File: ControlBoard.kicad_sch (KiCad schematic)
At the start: 1 part

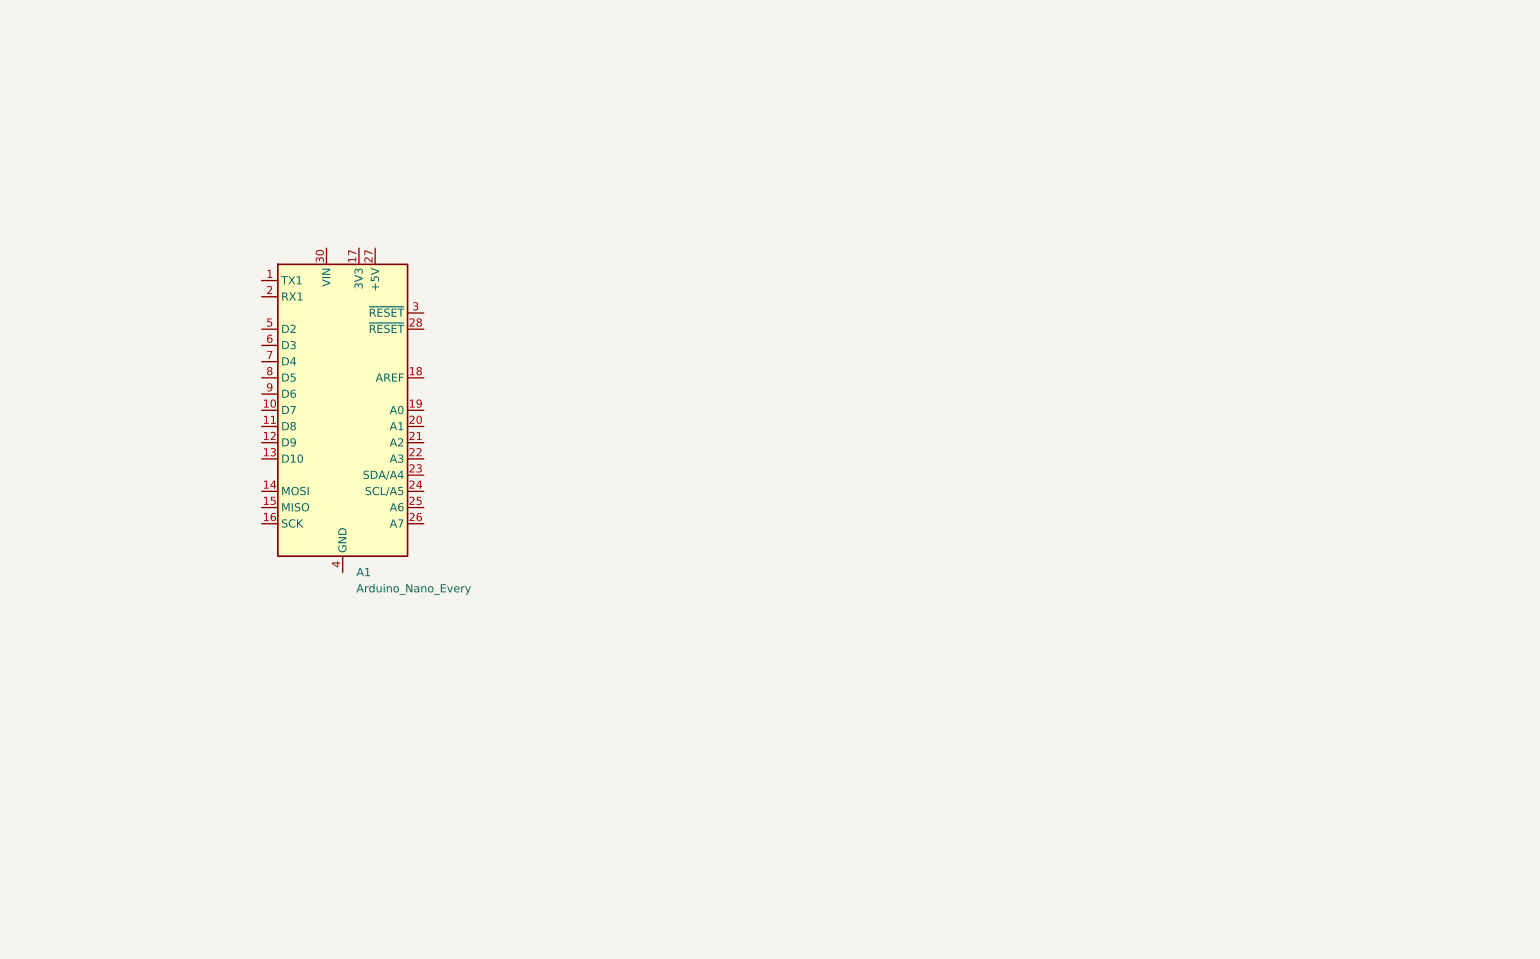
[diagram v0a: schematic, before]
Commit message: sync
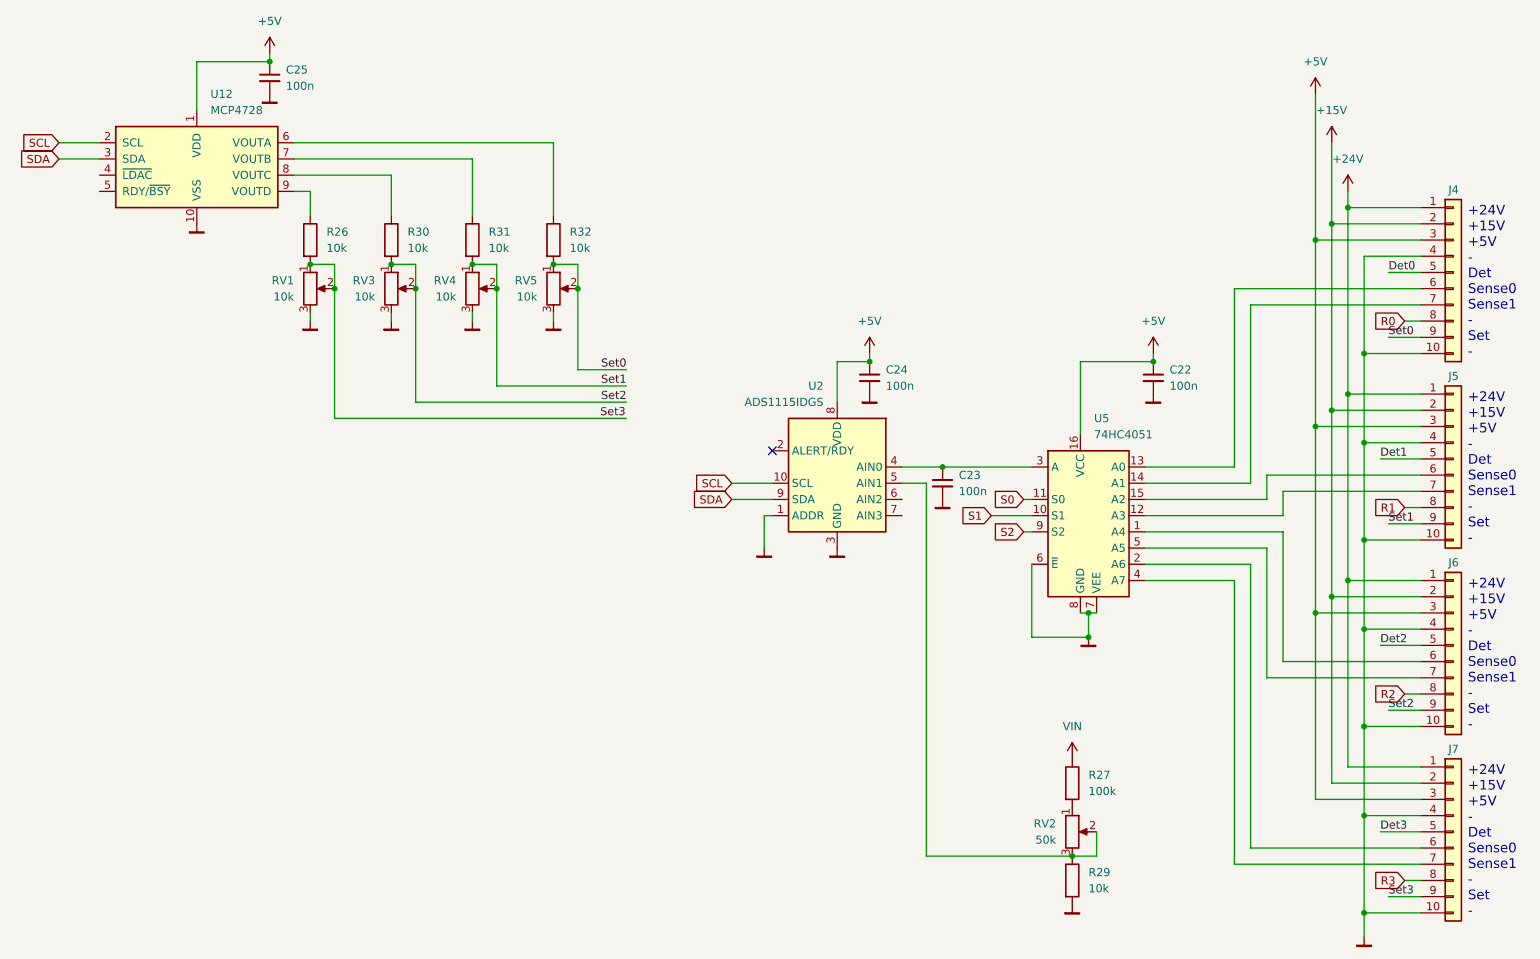
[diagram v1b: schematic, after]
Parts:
- removed A1: Arduino_Nano_Every, Module:Arduino_Nano, symbol MCU_Module:Arduino_Nano_Every
- added C22, C23, C24, C25: 100n, Capacitor_SMD:C_0603_1608Metric, symbol Device:C_Small
- added J4, J5, J6, J7: Conn_01x10, Connector_PinHeader_2.54mm:PinHeader_1x10_P2.54mm_Vertical, symbol Connector_Generic:Conn_01x10
- added R26, R29, R30, R31, R32: 10k, Resistor_SMD:R_0603_1608Metric, symbol Device:R
- added R27: 100k, Resistor_SMD:R_0603_1608Metric, symbol Device:R
- added RV1, RV3, RV4, RV5: 10k, Potentiometer_THT:Potentiometer_ACP_CA14-H5_Horizontal, symbol Device:R_Potentiometer
- added RV2: 50k, Potentiometer_THT:Potentiometer_ACP_CA14-H4_Horizontal, symbol Device:R_Potentiometer
- added U12: MCP4728, Package_SO:MSOP-10_3x3mm_P0.5mm, symbol Analog_DAC:MCP4728
- added U2: ADS1115IDGS, Package_SO:TSSOP-10_3x3mm_P0.5mm, symbol Analog_ADC:ADS1115IDGS
- added U5: 74HC4051, Package_SO:SOIC-16_3.9x9.9mm_P1.27mm, symbol 74xx:74HC4051
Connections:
- new net: J7.6 (Pin_6), U5.2 (A6)
- new net: J7.7 (Pin_7), U5.4 (A7)
- new net: R30.1, U12.8 (VOUTC)
- new net: R31.1, U12.7 (VOUTB)
- new net: R32.1, U12.6 (VOUTA)
- new net: R27.2, RV2.1
- new net: R29.1, RV2.2, RV2.3, U2.5 (AIN1)
- new net: R26.1, U12.9 (VOUTD)
- new net: J4.6 (Pin_6), U5.13 (A0)
- new net: J4.7 (Pin_7), U5.14 (A1)
- new net: C23.1, U2.4 (AIN0), U5.3 (A)
- new net: J6.6 (Pin_6), U5.1 (A4)
- new net: J5.7 (Pin_7), U5.12 (A3)
- new net: J5.6 (Pin_6), U5.15 (A2)
- new net: J6.7 (Pin_7), U5.5 (A5)
- new net +15V: J4.2 (Pin_2), J5.2 (Pin_2), J6.2 (Pin_2), J7.2 (Pin_2)
- new net +24V: J4.1 (Pin_1), J5.1 (Pin_1), J6.1 (Pin_1), J7.1 (Pin_1)
- new net +5V: C22.1, C24.1, C25.1, J4.3 (Pin_3), J5.3 (Pin_3), J6.3 (Pin_3), J7.3 (Pin_3), U12.1 (VDD), U2.8 (VDD), U5.16 (VCC)
- new net Det0: J4.5 (Pin_5)
- new net Det1: J5.5 (Pin_5)
- new net Det2: J6.5 (Pin_5)
- new net Det3: J7.5 (Pin_5)
- new net Masa: C22.2, C23.2, C24.2, C25.2, J4.10 (Pin_10), J4.4 (Pin_4), J5.10 (Pin_10), J5.4 (Pin_4), J6.10 (Pin_10), J6.4 (Pin_4), J7.10 (Pin_10), J7.4 (Pin_4), R29.2, RV1.3, RV3.3, RV4.3, RV5.3, U12.10 (VSS), U2.1 (ADDR), U2.3 (GND), U5.6 (~{E}), U5.7 (VEE), U5.8 (GND)
- new net R0: J4.8 (Pin_8)
- new net R1: J5.8 (Pin_8)
- new net R2: J6.8 (Pin_8)
- new net R3: J7.8 (Pin_8)
- new net S0: U5.11 (S0)
- new net S1: U5.10 (S1)
- new net S2: U5.9 (S2)
- new net SCL: U12.2 (SCL), U2.10 (SCL)
- new net SDA: U12.3 (SDA), U2.9 (SDA)
- new net Set0: J4.9 (Pin_9), R32.2, RV5.1, RV5.2
- new net Set1: J5.9 (Pin_9), R31.2, RV4.1, RV4.2
- new net Set2: J6.9 (Pin_9), R30.2, RV3.1, RV3.2
- new net Set3: J7.9 (Pin_9), R26.2, RV1.1, RV1.2
- new net VIN: R27.1
- no-connect marks 0 -> 1
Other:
- note added: "+24V +15V +5V - Det Sense0 Sense1 - Set -"
